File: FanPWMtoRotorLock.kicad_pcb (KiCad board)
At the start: 2 copper layers, 18.1 x 14.5 mm, 12 parts, among them J1 0022232031, J2 0022232031, Q2 MMBT2222A-7-F, Q3 MMBT2907ALT1G, U1 NE555P

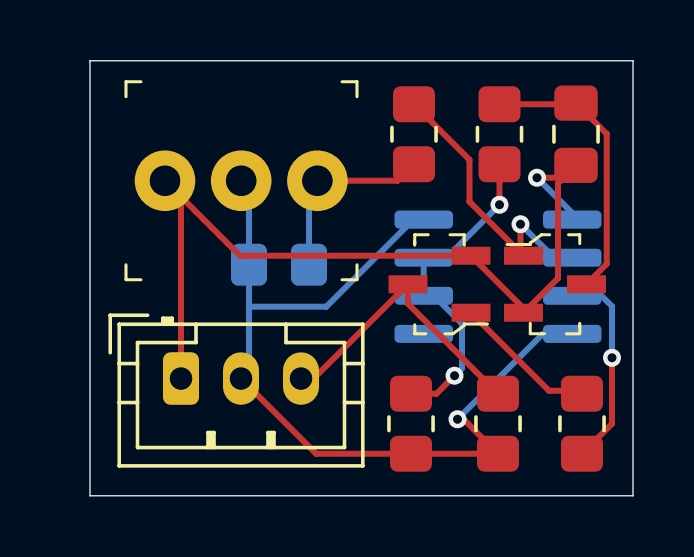
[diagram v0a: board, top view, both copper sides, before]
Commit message: Final layout, ready for manufacture
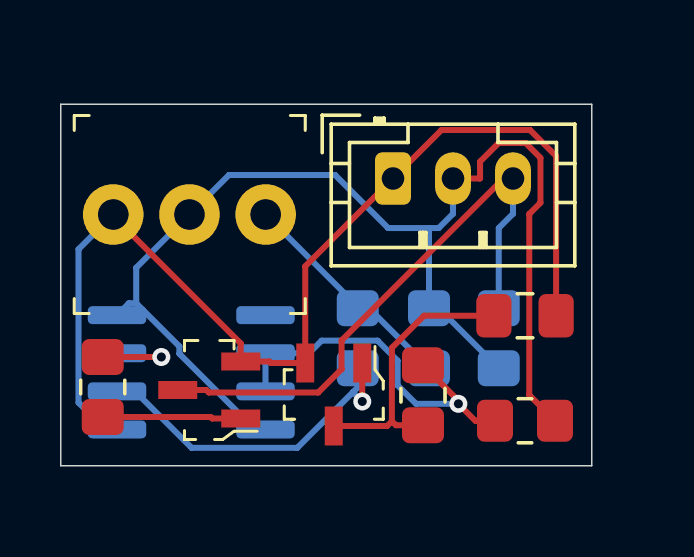
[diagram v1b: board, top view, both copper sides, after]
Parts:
- R2, R6: moved to B.Cu
- moved R5 16.0 mm to (116.4, 86.9), turned to -90 degrees
- moved U1 10.7 mm to (119.4, 86.4), turned to 0 degrees
- moved J2 9.72 mm to (126.1, 79.9)
- moved R4 9.07 mm to (127.1, 87.2), turned to -90 degrees
- moved Q2 8.45 mm to (120.0, 87.0)
- moved Q3 8.24 mm to (124.1, 87.1), turned to -90 degrees
- moved R2 7.05 mm to (124.9, 85.2), turned to -90 degrees
- moved C1 6.28 mm to (130.5, 84.5), turned to 0 degrees
- moved R1 5.57 mm to (127.3, 85.2), turned to -90 degrees
- moved R3 3.80 mm to (130.5, 88.0), turned to 180 degrees
- moved R6 2.85 mm to (129.6, 85.2)
- moved J1 2.06 mm to (116.8, 81.1)
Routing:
- net Net-(U1-R): track 30.6 -> 41.2 mm, vias 1 -> 0
- net Net-(Q2-C): track 9.76 -> 19.2 mm
- net Net-(Q2-E): track 29.7 -> 36.4 mm, vias 1 -> 0
- net Net-(U1-Q): track 6.80 -> 3.48 mm
- net Net-(Q3-B): track 9.84 -> 12.0 mm
- net Net-(U1-DIS): track 11.1 -> 12.5 mm, vias 2 -> 1
- net Net-(J1-Pad3): track 6.36 -> 7.60 mm
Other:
- board size 18.1 x 14.5 mm -> 17.7 x 12 mm
